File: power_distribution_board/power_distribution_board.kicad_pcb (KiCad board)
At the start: 2 copper layers, 144 x 88 mm, 72 parts, among them J1 CONN_01x03, J10 CONN_02X01, J11 CONN_02X01, J12 CONN_02X01, J13 CONN_02X01, J14 CONN_02X01, J15 CONN_02X01, J16 CONN_02X01, J17 CONN_02X01, J18 CONN_02X01, J19 CONN_02X01, J2 CONN_02X01, J20 CONN_02X01, J21 CONN_02X01, J22 CONN_02X01, J23 CONN_02X01, J3 CONN_02X01, J4 CONN_02X01, J5 CONN_02X01, J6 CONN_02X01, J7 CONN_02X01, J8 CONN_02X01, J9 CONN_02X01, Q1 NMOS_SSSGD, Q2 NMOS_SSSGD, Q3 NMOS_SSSGD, Q4 NMOS_SSSGD, Q5 Q_NMOS_GSD, U1 EHHD015A0A, U2 LTC1473, U3 EHHD010A0B, U4 LM317EMP, U5 BTS6133D, U6 A1120

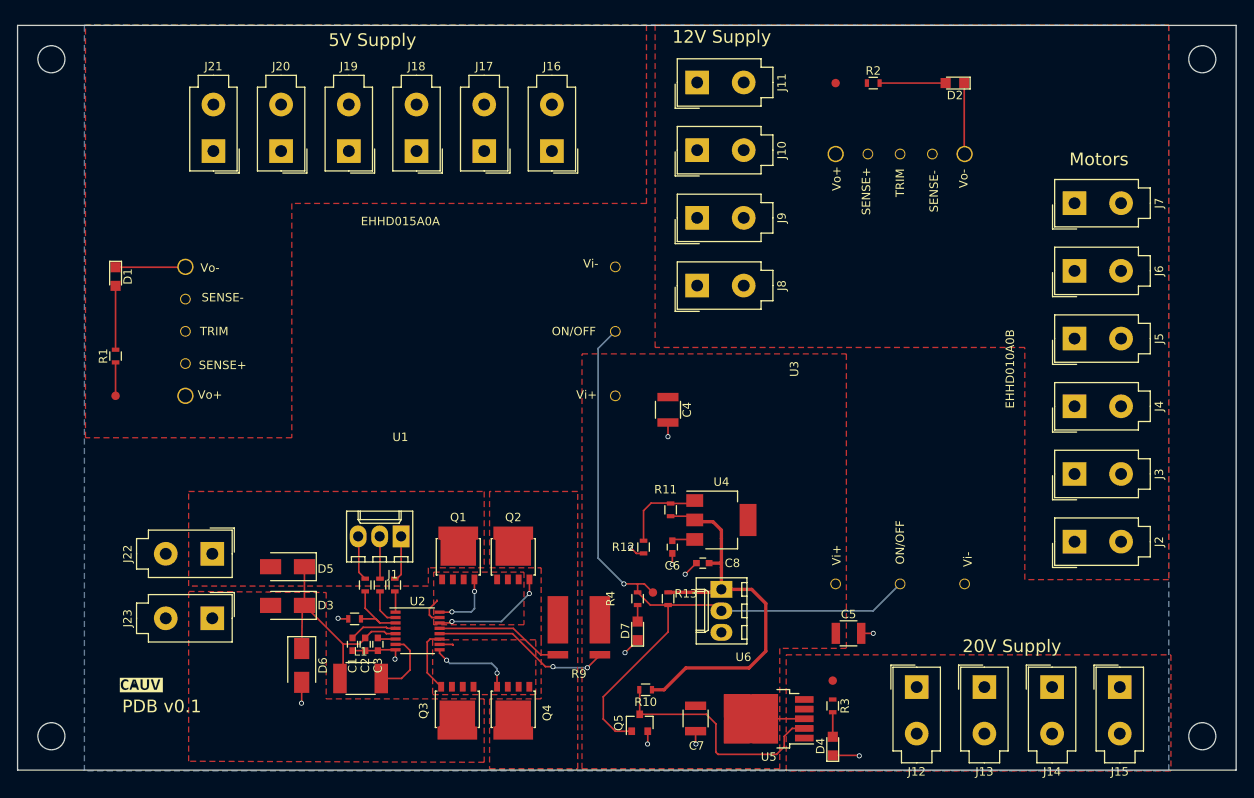
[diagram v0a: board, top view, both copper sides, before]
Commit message: final modifications
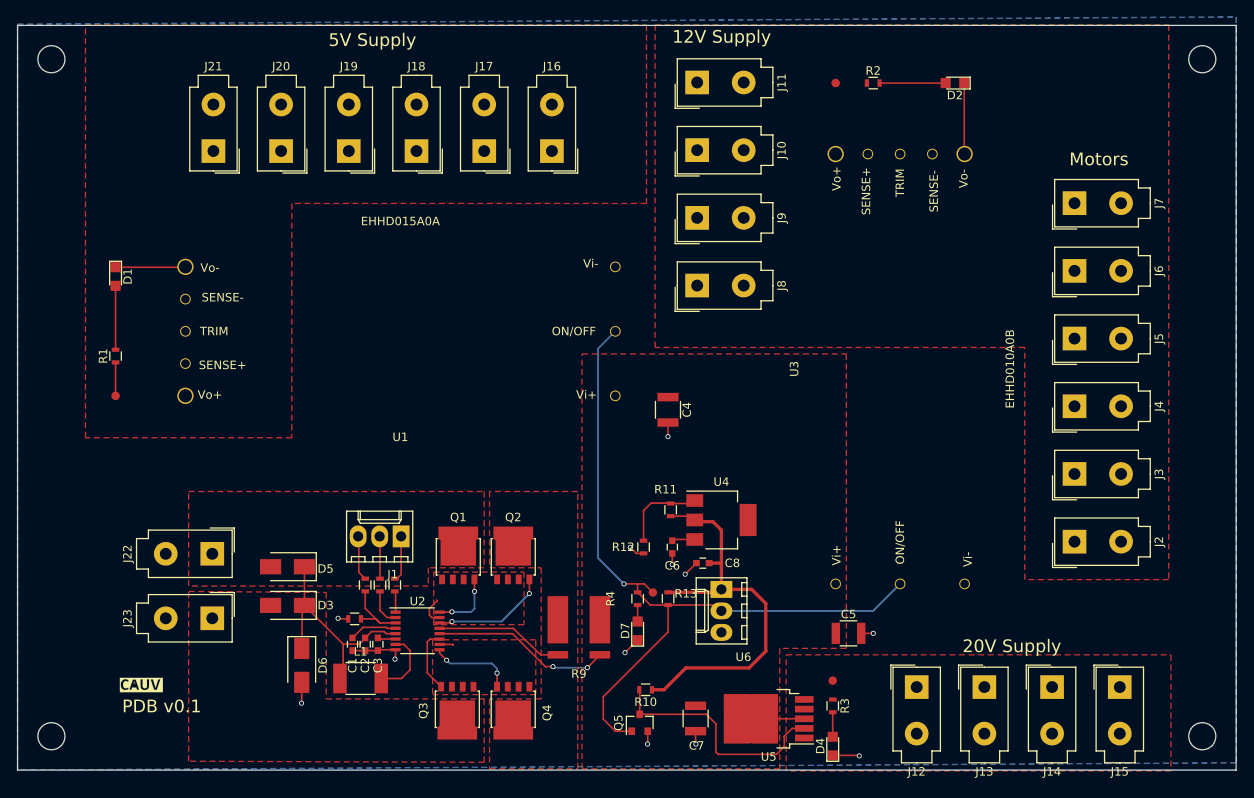
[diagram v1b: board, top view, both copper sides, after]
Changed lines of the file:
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@@
-(kicad_pcb (version 4) (host pcbnew 4.0.7)
+(kicad_pcb (version 4) (host pcbnew 4.0.6)
   (general
     (links 201)
     (no_connects 0)
-    (area 72.924999 60.924999 217.075001 149.075001)
+    (area 72.924999 59.825 217.075001 150.275)
     (thickness 1.6)
     (drawings 9)
@@
     (polygon
       (pts
-        (xy 209.042 149.098) (xy 80.899 149.098) (xy 80.899 60.96) (xy 209.042 60.96)
+        (xy 217 148.138) (xy 73 149) (xy 73 60.862) (xy 217 60)
       )
     )
